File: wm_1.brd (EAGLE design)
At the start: 160 x 100 mm, 25 parts, among them IC1 TINY13-20MM0, IC2 DS1813-SMD, T1 MMBT3904, T2 BT138-V

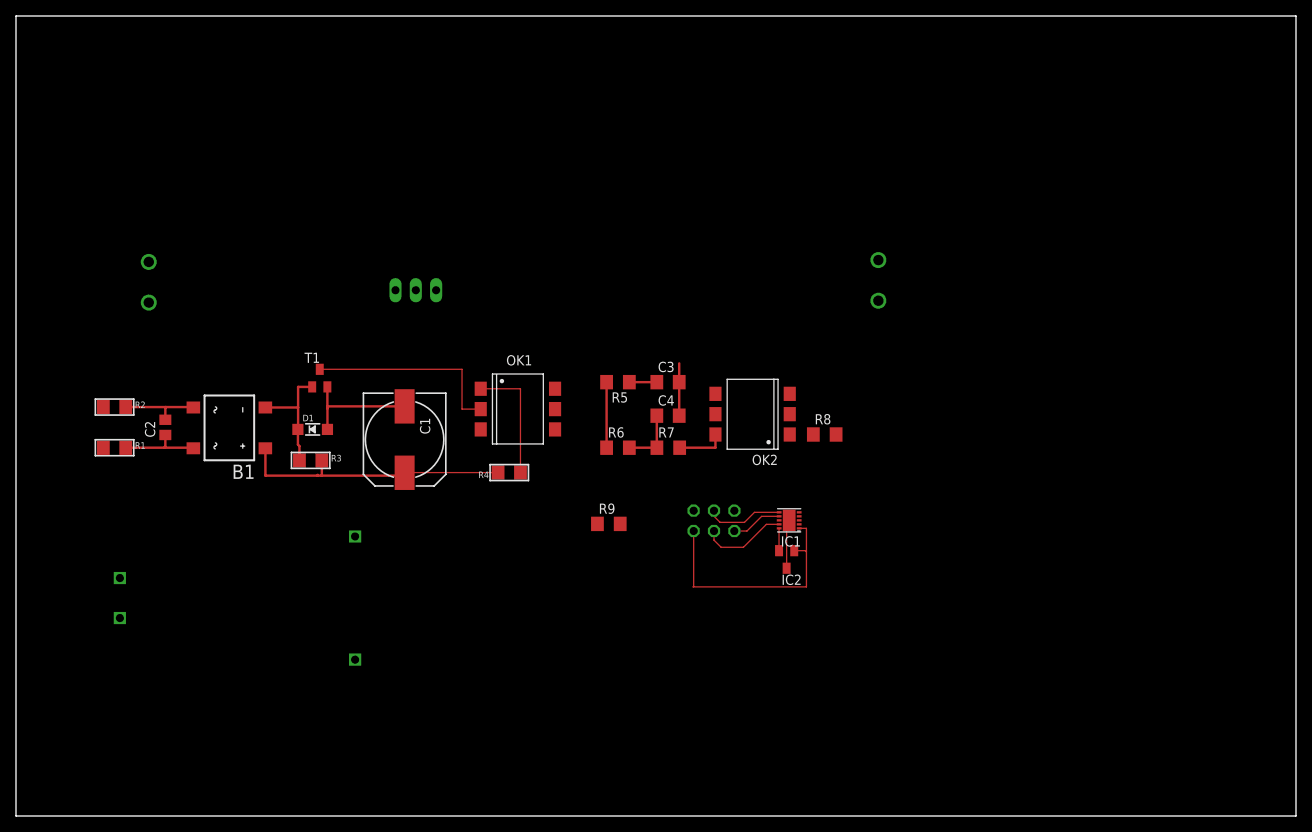
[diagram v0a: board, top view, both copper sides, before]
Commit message: wip
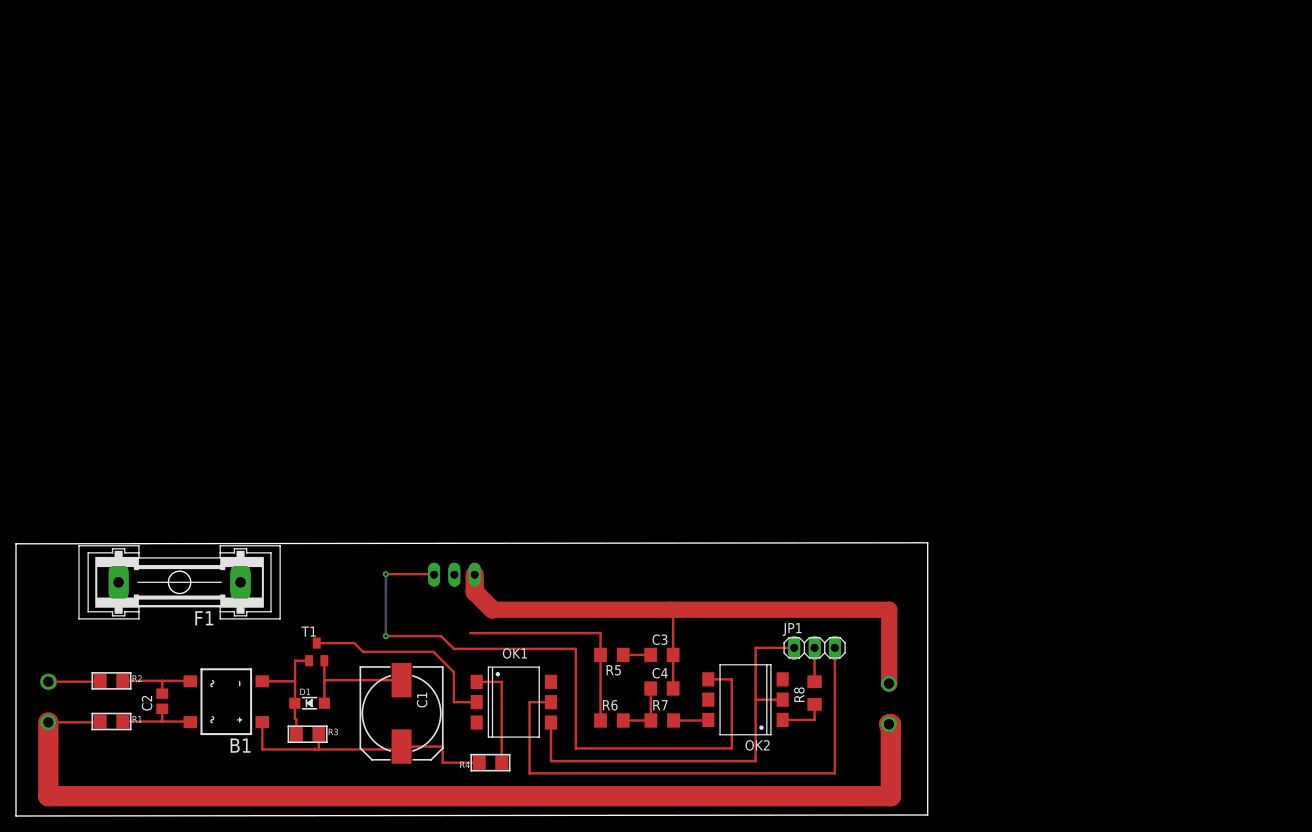
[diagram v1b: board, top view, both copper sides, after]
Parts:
- removed HLK1: HLK-PM013W, hi-link:HLK-PM01
- removed IC1: TINY13-20MM0, atmel:10M1
- removed IC2: DS1813-SMD, MyLib:SOT-23
- removed R9: 1k, rcl:R1206
- added F1: (no value), fuse:GSH15
- JP1: device pinhead:2X03 -> pinhead:1X03
- moved IN 54.0 mm to (4.06, 14.2), turned to 270 degrees
- moved OUT 52.9 mm to (109.1, 14.0), turned to 90 degrees
- moved OK1 36.6 mm to (62.2, 14.2)
- moved R4 36.3 mm to (59.3, 6.67)
- moved T2 35.9 mm to (54.8, 32.7)
- moved OK2 35.7 mm to (91.2, 14.5)
- moved B1 34.2 mm to (26.3, 14.3)
- moved C1 34.2 mm to (48.2, 12.8)
- moved C2 34.2 mm to (18.3, 14.4)
- moved D1 34.2 mm to (36.7, 14.1)
- moved R1 34.2 mm to (11.9, 11.8)
- moved R2 34.2 mm to (11.9, 16.9)
- moved R3 34.2 mm to (36.4, 10.2)
- moved T1 34.2 mm to (37.6, 20.5)
- moved C3 34.1 mm to (80.7, 20.1)
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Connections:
- net N$9 renamed GATE
- removed net +5V: HLK1.P$4, IC1.10, IC2.2, JP1.2, R9.1
- removed net MISO: IC1.7, JP1.1
- removed net MOSI: IC1.6, JP1.4
- removed net RESET: IC1.1, IC2.1, JP1.5
- removed net SCK: IC1.9, JP1.3
- new net N$9: F1.2, IN.1
- net GND: now also JP1.1; no longer HLK1.P$3, IC1.11, IC1.5, IC2.3, JP1.6
- net GROUND: now also R1.1; no longer HLK1.P$2, R2.1
- net HOT: now also F1.1, R2.1; no longer HLK1.P$1, IN.1, R1.1
- net ON/OFF: now also JP1.2; no longer IC1.4
- net ZERO: now also JP1.3; no longer R9.2
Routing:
- net GROUND: track 0.11 -> 130.4 mm
- net GATE: track 0.00 -> 81.9 mm, vias 0 -> 2
- net LOAD: track 6.54 -> 74.3 mm
- net ZERO: track 0.00 -> 65.4 mm
- net GND: track 6.12 -> 52.8 mm
- net RESET: track 31.0 -> 0.00 mm
- net HOT: track 8.28 -> 33.8 mm
- net SCK: track 10.8 -> 0.00 mm
- net MOSI: track 9.68 -> 0.00 mm
- net MISO: track 6.37 -> 0.00 mm
- net N$17: track 0.28 -> 6.22 mm
- net ON/OFF: track 0.00 -> 4.23 mm
- net +5V: track 2.80 -> 0.00 mm
- net N$6: track 15.4 -> 13.2 mm
- net N$16: track 6.12 -> 4.41 mm
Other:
- board size 160 x 100 mm -> 114 x 34.2 mm
